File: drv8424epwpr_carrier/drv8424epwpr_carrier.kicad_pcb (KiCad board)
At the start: 2 copper layers, 27 parts, among them J1 Input_01x08, J2 Output_01x08, J3 POW_01x02, U1 DRV8424EPWPR, U2 DMP4013LFG-7

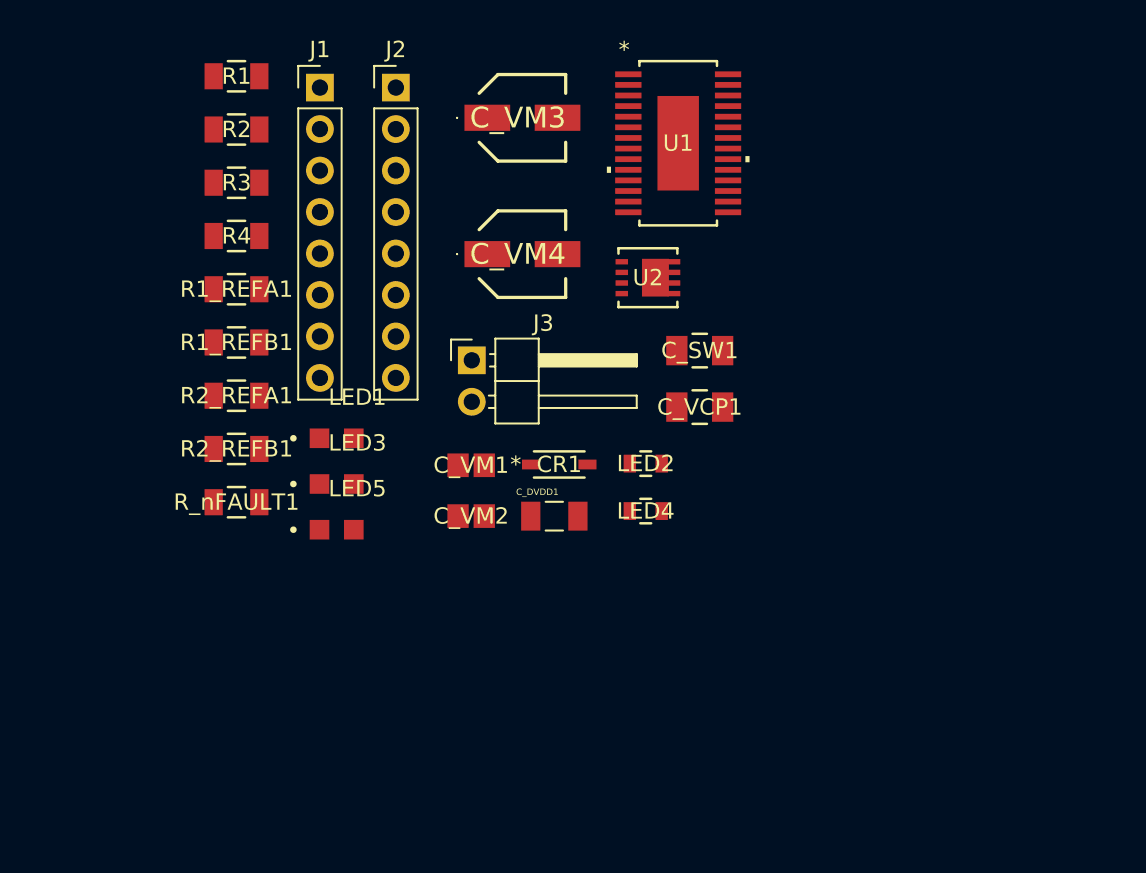
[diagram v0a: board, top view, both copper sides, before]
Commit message: update layout
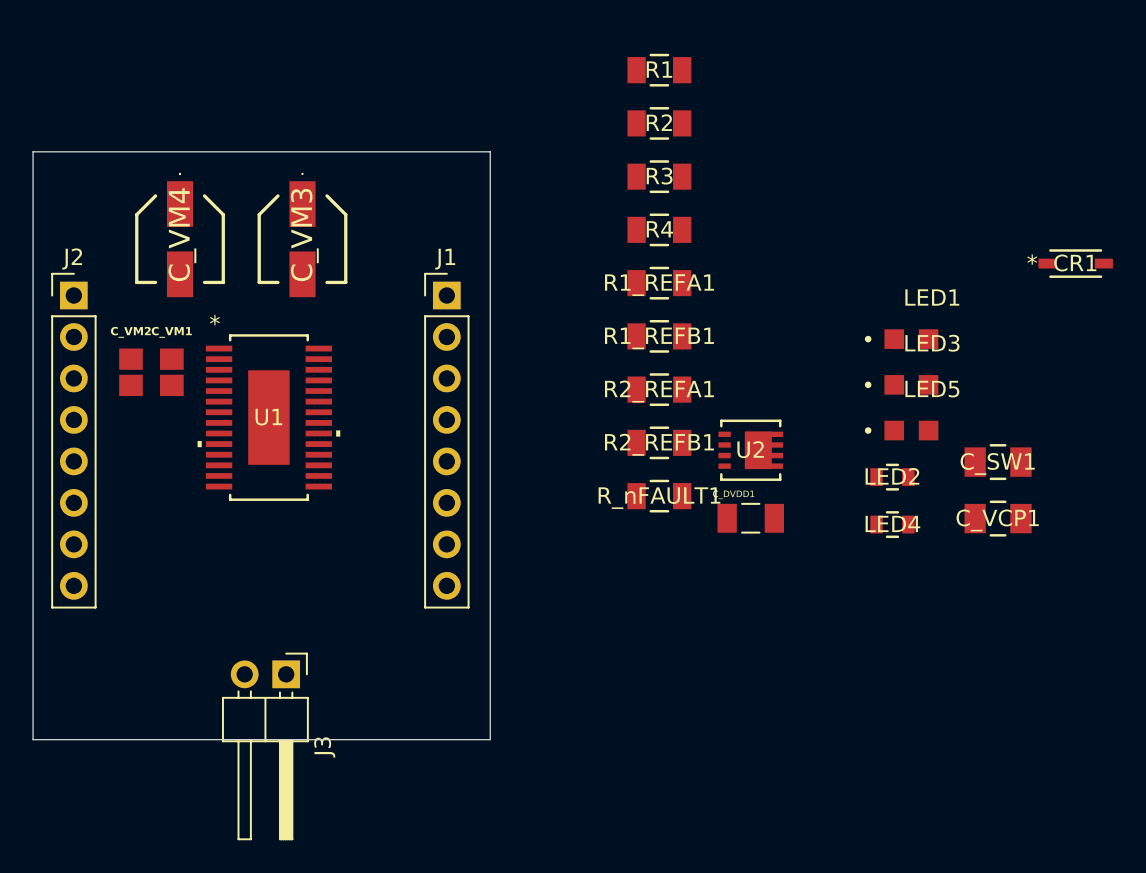
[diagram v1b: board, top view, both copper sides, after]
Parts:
- moved LED1 35.7 mm to (103.8, 61.5)
- moved LED3 35.7 mm to (103.8, 64.3)
- moved LED5 35.7 mm to (103.8, 67.1)
- moved CR1 33.9 mm to (113.9, 56.8)
- moved U1 30.2 mm to (64.4, 66.3)
- moved R1 25.9 mm to (88.4, 45.0)
- moved R1_REFA1 25.9 mm to (88.4, 58.0)
- moved R1_REFB1 25.9 mm to (88.4, 61.3)
- moved R2 25.9 mm to (88.4, 48.3)
- moved R2_REFA1 25.9 mm to (88.4, 64.6)
- moved R2_REFB1 25.9 mm to (88.4, 67.8)
- moved R3 25.9 mm to (88.4, 51.5)
- moved R4 25.9 mm to (88.4, 54.8)
- moved R_nFAULT1 25.9 mm to (88.4, 71.1)
- moved J2 23.5 mm to (52.5, 58.8)
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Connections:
- J1 pad 1: +3V3 -> NSLEEP
- J1 pad 2: GND -> AEN
- J1 pad 3: NFAULT -> APH
- J1 pad 4: NSLEEP -> BEN
- J1 pad 5: AEN -> BPH
- J1 pad 6: APH -> NFAULT
- J1 pad 7: BEN -> GND
- J1 pad 8: BPH -> +3V3
- J2 pad 7: BOUT2 -> BOUT1
- J2 pad 8: BOUT1 -> BOUT2
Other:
- board outline added: 28 x 36 mm

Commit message: update layout
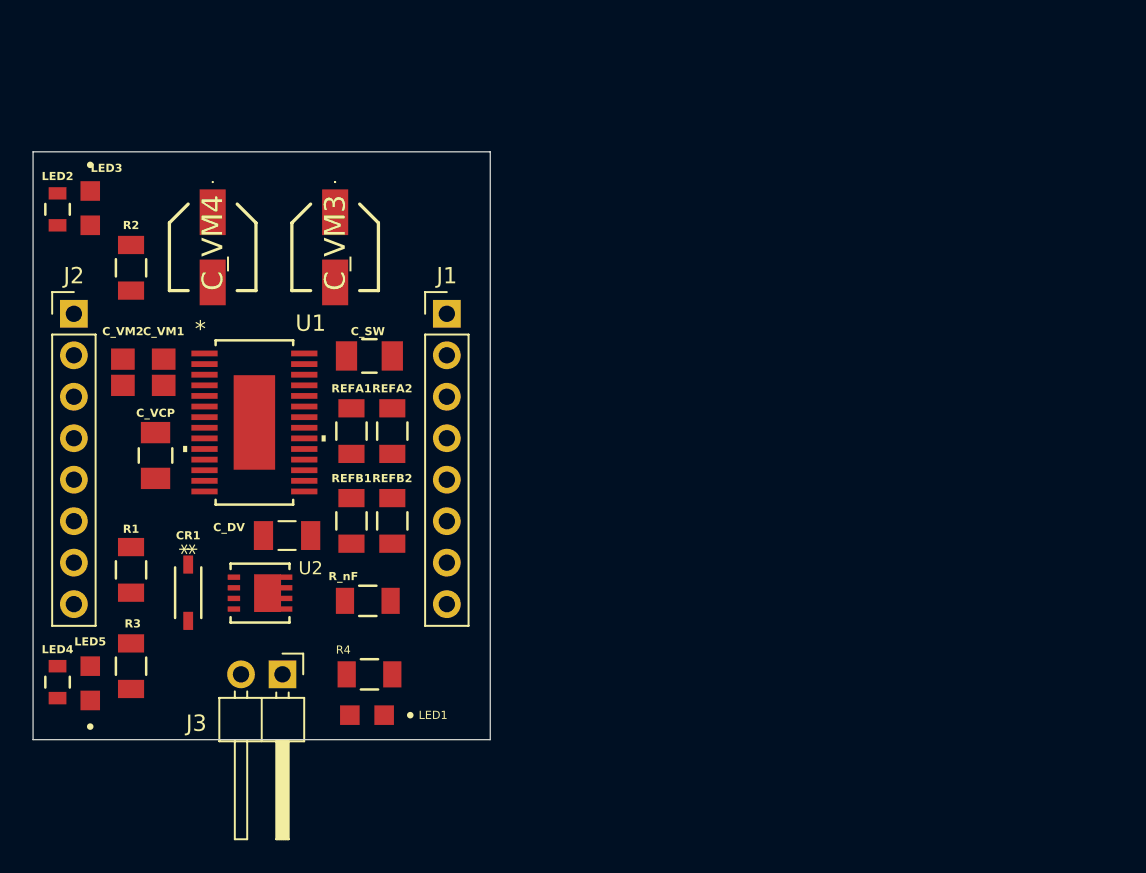
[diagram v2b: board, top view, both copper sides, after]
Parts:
- LED1: value YELLOW -> YLW
- LED2, LED4: value GREEN -> GRN
- moved CR1 58.0 mm to (59.5, 77.0), turned to -90 degrees
- moved LED2 53.7 mm to (51.5, 53.5), turned to 90 degrees
- moved LED5 52.6 mm to (53.5, 82.5), turned to 90 degrees
- moved LED4 52.0 mm to (51.5, 82.5), turned to -90 degrees
- moved C_VCP 51.7 mm to (57.5, 68.6), turned to -90 degrees
- moved LED3 51.4 mm to (53.5, 53.5), turned to -90 degrees
- moved R1 44.5 mm to (56.0, 75.6), turned to 90 degrees
- moved R3 44.1 mm to (56.0, 81.5), turned to -90 degrees
- moved LED1 40.5 mm to (70.5, 84.5), turned to 180 degrees
- moved C_SW 39.0 mm to (70.6, 62.5)
- moved R2 33.5 mm to (56.0, 57.1), turned to 90 degrees
- moved R4 32.5 mm to (70.6, 82.0), turned to 180 degrees
- moved U2 31.3 mm to (63.9, 77.0)
- moved C_DV 28.4 mm to (65.6, 73.5), turned to 180 degrees
- moved REFB1 22.0 mm to (69.5, 72.6), turned to 90 degrees
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- renumbered C_DVDD1 to C_DV, C_SW1 to C_SW, C_VCP1 to C_VCP, R1_REFA1 to REFA1, R2_REFA1 to REFA2, R1_REFB1 to REFB1, R2_REFB1 to REFB2, R_nFAULT1 to R_nF
